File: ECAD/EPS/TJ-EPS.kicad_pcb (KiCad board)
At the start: 2 copper layers, 449 parts, among them J1 SWD, J2 BOOT, J3 S1A, J4 S1B, J5 S2A, J6 S2B, J7 S3A, J8 S3B, J9 TELEM_IN, Q1 2N7002, Q10 SIR167DP, Q11 SIR167DP, Q12 2N7002, Q13 IRF7458, Q14 2N7002, Q15 2N7002, Q16 2N7002, Q17 IRF7458, Q18 IRF7458, Q19 2N7002, Q2 IRF7425, Q20 2N7002, Q21 2N7002, Q22 2N7002, Q23 2N7002, Q24 2N7002, Q25 2N7002, Q26 2N7002, Q27 2N7002, Q28 IRF7458, Q29 2N7002, Q3 IRF7425, Q30 IRF7458, Q31 2N7002, Q32 IRF7458, Q33 2N7002, Q34 IRF7458, Q35 2N7002, Q36 IRF7458, Q37 2N7002, Q38 IRF7458, Q39 2N7002, Q4 IRF7458, Q40 IRF7458, Q41 2N7002, Q42 IRF7458, Q43 2N7002, Q44 IRF7458, Q45 2N7002, Q46 IRF7458, Q47 2N7002, Q48 IRF7458, Q49 2N7002, Q5 IRF7458, Q50 IRF7458, Q6 Si4186DY, Q7 IRF7458, Q8 2N7002, Q9 IRF7458, SW1 INHIBIT 1, SW2 INHIBIT 2, SW3 INHIBIT 3, U1 CD74HC4067SM, U10 L78L33_SO8, U11 MCP4812, U12 MCP4812, U13 LT6106, U14 LT6106, U15 LM358, U16 LT3652EMSE, U17 LT6106, U18 LT6106, U19 LM358, U2 CD74HC4067SM, U20 LT3652EMSE, U21 LM358, U22 LT6106, U23 LT6106, U24 LT3652EMSE, U25 LMC555xM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

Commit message: inhibit resistor values, among other things
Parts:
- Q2, Q3: value IRF7425 -> IRF7458

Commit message: Restandardize stack headers a bit
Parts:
- R10, R12, R63: value 10K -> 100K
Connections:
- H1 pad 10: GND -> SW2
- H1 pad 11: SW1 -> SW3
- H1 pad 12: SW2 -> SW4
- H1 pad 13: SW3 -> SW5
- H1 pad 14: SW4 -> SW6
- H1 pad 15: SW6 -> SW7
- H1 pad 16: SW5 -> SW8
- H1 pad 17: SW8 -> SW9
- H1 pad 18: SW7 -> SW10
- H1 pad 19: SW10 -> SW11
- H1 pad 20: SW9 -> SW12
- H1 pad 21: SW12 -> GND
- H1 pad 22: SW11 -> GND
- H1 pad 23: GND -> (no net)
- H1 pad 24: GND -> (no net)
- H1 pad 25: +BATT -> +5V
- H1 pad 26: +BATT -> +5V
- H1 pad 27: +5V -> +3V3
- H1 pad 28: +5V -> +3V3
- H1 pad 29: +3V3 -> GND
- H1 pad 30: +3V3 -> GND
- H1 pad 39: BCR_OUT -> (no net)
- H1 pad 40: BCR_OUT -> (no net)
- H1 pad 43: GND -> BCR_OUT
- H1 pad 44: GND -> BCR_OUT
- H1 pad 45: VUSB -> +BATT
- H1 pad 46: VUSB -> +BATT
- H1 pad 9: GND -> SW1
- H2 pad 30: /SCK -> (no net)
- H2 pad 32: /MISO -> VUSB
- H2 pad 33: (no net) -> /SCK
- H2 pad 34: /MOSI -> (no net)
- H2 pad 35: (no net) -> /MISO
- H2 pad 36: /SS -> (no net)
- H2 pad 37: (no net) -> /MOSI
- H2 pad 39: (no net) -> /SS
- H2 pad 41: (no net) -> /SDA
- H2 pad 42: /SDA -> (no net)
- H2 pad 43: (no net) -> /SCL
- H2 pad 44: /SCL -> (no net)
- R10 pad 1: /SolarConditioning/MPPT1/VOUT -> Net-(Q4-Pad4)
- R10 pad 2: Net-(Q4-Pad4) -> GND
- R11 pad 1: Net-(Q4-Pad4) -> /SolarConditioning/MPPT1/VOUT
- R12 pad 1: Net-(Q4-Pad5) -> Net-(Q5-Pad4)
- R12 pad 2: Net-(Q5-Pad4) -> GND
- R13 pad 1: Net-(Q5-Pad4) -> Net-(Q4-Pad5)
- R63 pad 1: PCM_IN -> Net-(Q7-Pad4)
- R63 pad 2: Net-(Q7-Pad4) -> GND
- R64 pad 1: Net-(Q7-Pad4) -> PCM_IN
- SW1 pad 2: GND -> Net-(Q4-Pad4)
- SW2 pad 2: GND -> Net-(Q5-Pad4)
- SW3 pad 2: GND -> Net-(Q7-Pad4)

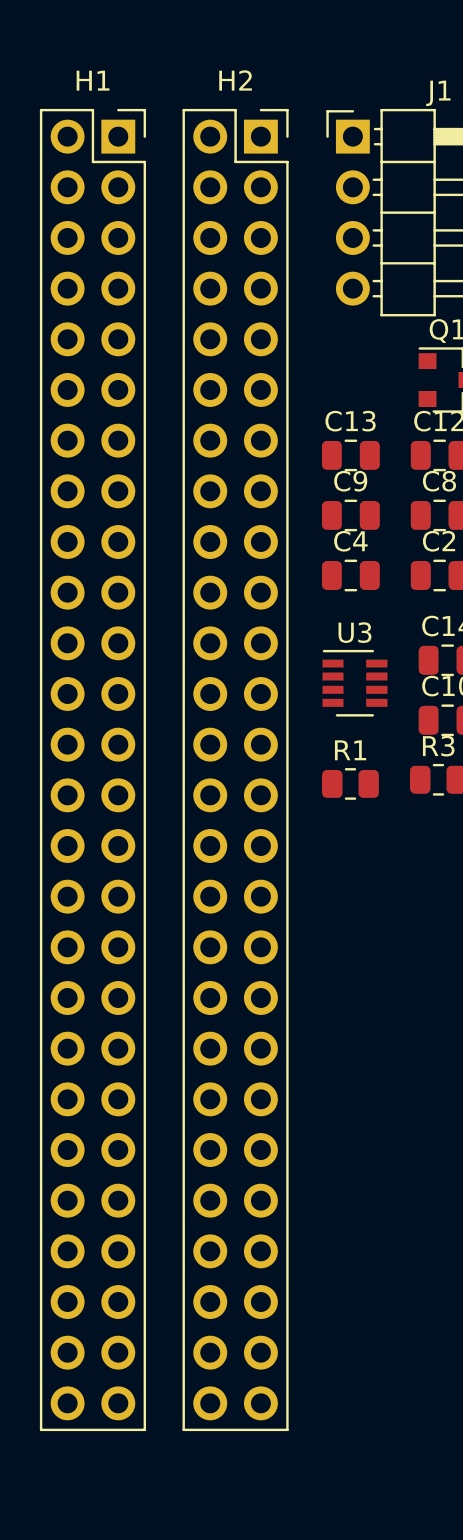
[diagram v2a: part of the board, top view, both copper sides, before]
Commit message: replace stack header footprint
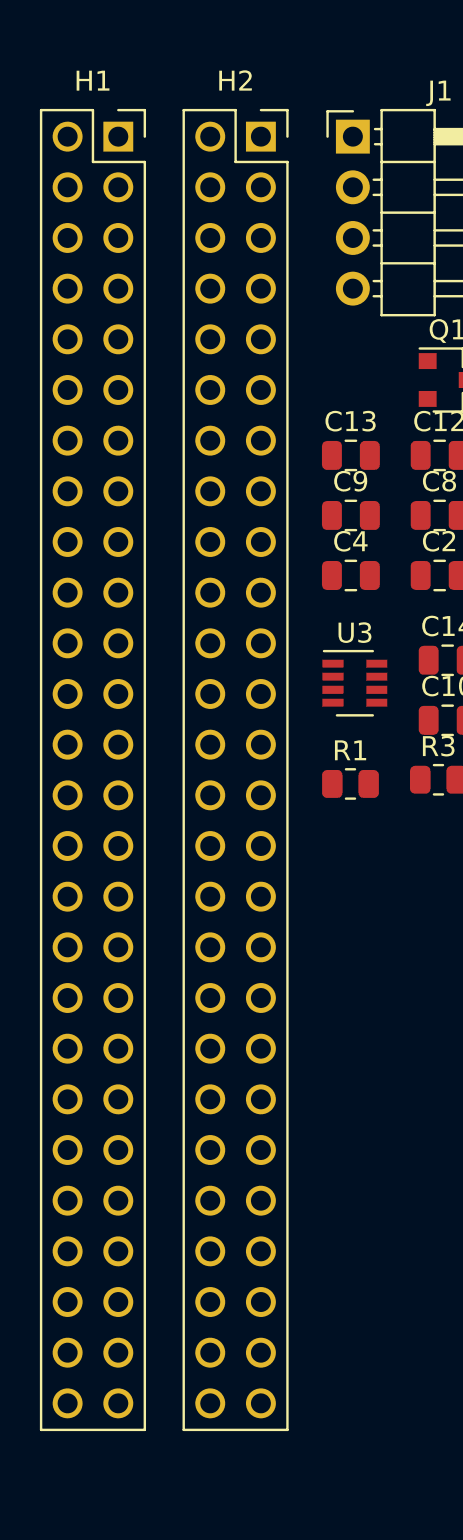
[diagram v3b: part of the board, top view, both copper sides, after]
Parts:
- H1, H2: footprint Connector_PinSocket_2.54mm:PinSocket_2x26_P2.54mm_Vertical -> footprints:PinSocket_2x26_P2.54mm_Vertical
